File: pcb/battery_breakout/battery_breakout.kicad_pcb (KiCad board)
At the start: 2 copper layers, 12.8 x 77 mm, 5 parts, among them J1 BATTERY_HOLDER, J2 CONN_01x02, J3 CONN_01x02, J4 BATTERY_HOLDER, X1 Mount

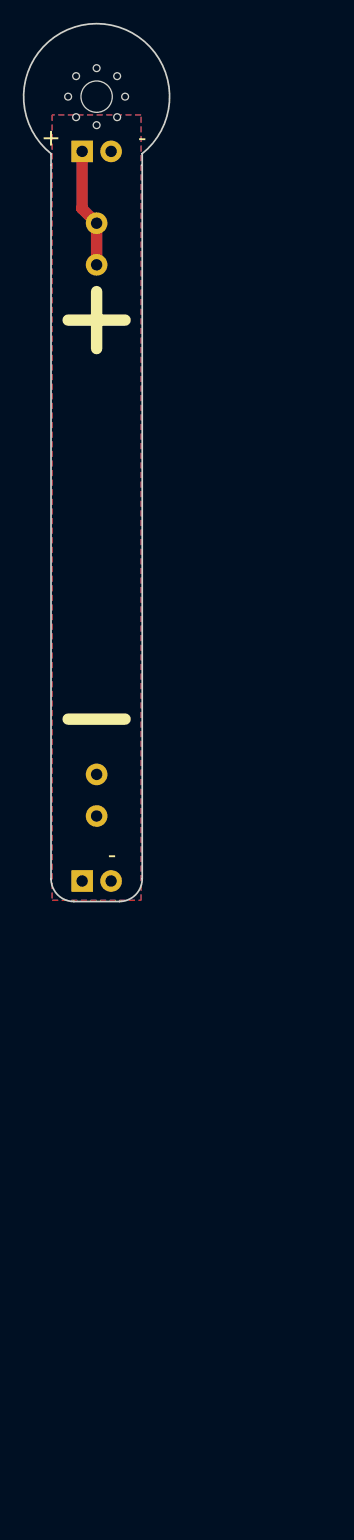
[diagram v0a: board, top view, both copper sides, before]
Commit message: Fix small changes to both boards
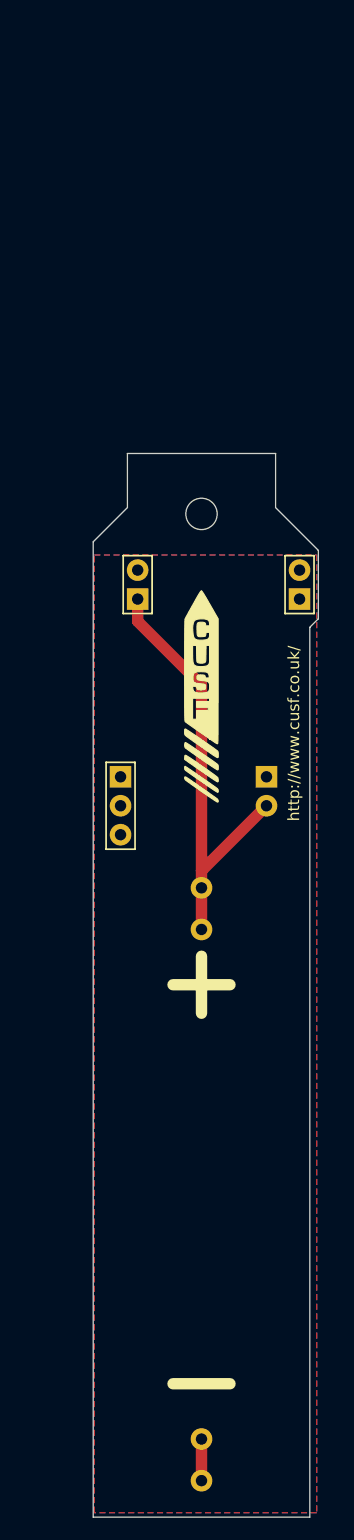
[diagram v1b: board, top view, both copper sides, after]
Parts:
- removed X1: Mount, agg:M2.5_MOUNT
- added G***: LOGO, jerboa:cusf_logo, F.Cu at (149.2, 110.0)
- added REF**: SIL-254P-03, agg:SIL-254P-03, F.Cu at (142.1, 119.6)
- added REF**: SIL-254P-02, agg:SIL-254P-02, F.Cu at (157.8, 100.2)
- added REF**: M2.5_HOLE, agg:M2.5_HOLE, F.Cu at (149.2, 94.0)
- J3: moved to F.Cu
- moved J1 59.0 mm to (149.2, 152.8)
- moved J4 59.0 mm to (149.2, 152.8)
- moved J2 58.1 mm to (154.9, 118.3), turned to 270 degrees
- moved J3 26.2 mm to (143.6, 100.2), turned to 90 degrees
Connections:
- J2 pad 1: /V_BATT -> Net-(J2-Pad1)
- J2 pad 2: GND -> /V_BATT
- J3 pad 1: (no net) -> /V_BATT
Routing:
- net /V_BATT: track 10.5 -> 39.4 mm
- net GND: track 0.00 -> 3.65 mm
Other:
- board size 12.8 x 77 mm -> 19.8 x 93.3 mm
- board text added: "Feb 2019"
- board text added: "Jerboa Battery"
- board text added: "Joel Mayer"
- board text added: "VBATT"
- board text added: "VSOLAR"
- board text added: "http://www.cusf.co.uk/"
- board text removed: "+"
- board text removed: "-"

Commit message: Make some last minute changes to PCBs before sending off for manufacture
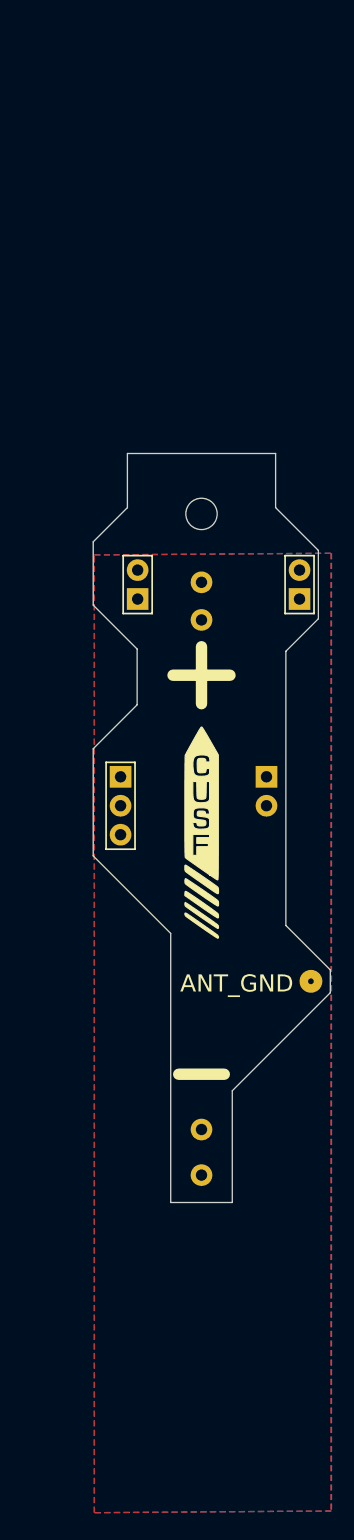
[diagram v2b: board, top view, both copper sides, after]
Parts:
- added TP1: TESTPAD, jerboa:ANT_GND_PASSTHROUGH, F.Cu at (158.4, 126.9)
- J1: footprint battery_breakout:AAA_battery_holder -> jerboa:AAA_battery_holder
- J4: footprint battery_breakout:AA_battery_holder -> jerboa:AA_battery_holder
- moved J1 27.2 mm to (149.2, 125.7)
- moved J4 26.8 mm to (149.2, 126.0)
- moved G*** 11.9 mm to (149.2, 122.0)
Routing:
- net /V_BATT: track 39.4 -> 0.00 mm
- net GND: track 3.65 -> 0.00 mm
- added copper zone on F.Cu, net /V_BATT
- removed copper zone on F.Cu, net GND
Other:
- board size 19.8 x 93.3 mm -> 20.8 x 65.7 mm
- board text added: "+"
- board text added: "-"
- board text added: "ANT_GND"
- board text removed: "http://www.cusf.co.uk/"
